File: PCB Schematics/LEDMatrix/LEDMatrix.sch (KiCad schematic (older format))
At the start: 25 parts, among them J1 Conn_01x02, P1 Digital, SW1 SW_Push, SW2 SW_Push, SW3 SW_Push, SW4 SW_Push, SW5 SW_Push, U1 74HC595, U2 74HC595, U3 LED8x8Matrix, U4 LED8x8Matrix

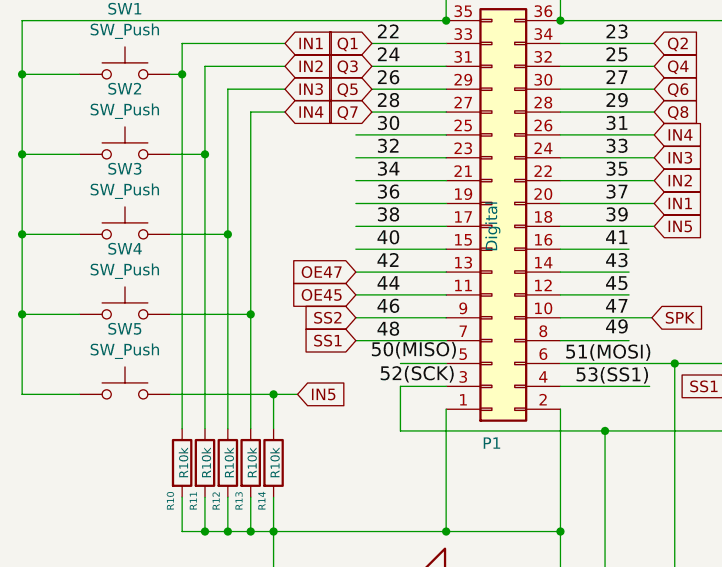
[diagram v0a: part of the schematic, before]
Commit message: Changed drawings
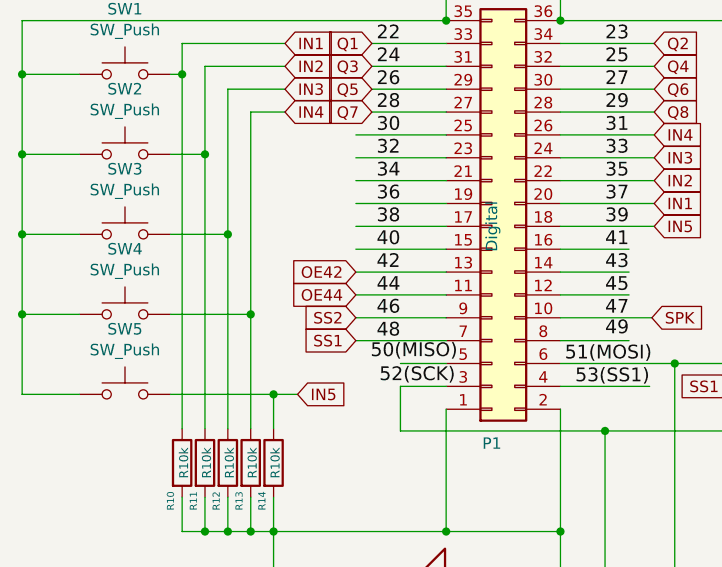
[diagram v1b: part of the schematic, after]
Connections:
- net labels added: OE42, OE44
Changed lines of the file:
@@
 EESchema Schematic File Version 4
-LIBS:LEDMatrix-cache
-EELAYER 29 0
+EELAYER 30 0
 EELAYER END
 $Descr A4 11693 8268
@@
 $EndComp
 Text GLabel 2555 3230 0    50   Input ~ 0
-OE45
+OE44
 Text GLabel 2555 3130 0    50   Input ~ 0
-OE47
+OE42
 Text GLabel 2555 3330 0    50   Input ~ 0
 SS2
